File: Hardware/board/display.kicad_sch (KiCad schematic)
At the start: 1 part, among them U4 HS35B01A

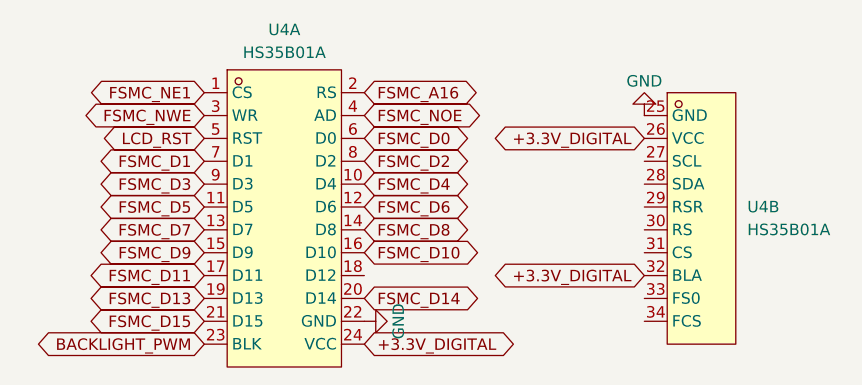
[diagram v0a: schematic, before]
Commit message: i am cooked
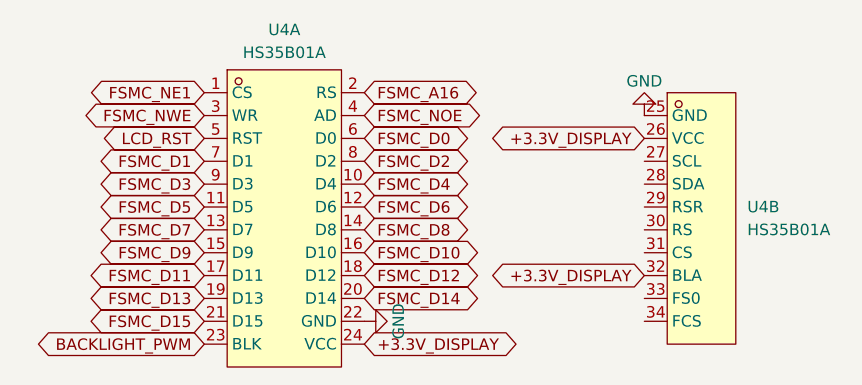
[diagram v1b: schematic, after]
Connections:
- net FSMC_D12: now reaches U4.18 (D12)
- net +3.3V_DIGITAL renamed +3.3V_DISPLAY
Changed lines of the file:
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@@
 	(generator_version "10.0")
 	(paper "A4")
+	(global_label "+3.3V_DISPLAY"
+		(shape bidirectional)
+		(at 146.05 51.435 180)
+		(effects
+			(font
+				(size 1.27 1.27)
+			)
+			(justify right)
+		)
+		(property "Intersheetrefs" "${INTERSHEET_REFS}"
+			(at 146.05 51.435 0)
+			(hide yes)
+			(show_name no)
+			(do_not_autoplace no)
+			(effects
+				(font
+					(size 1.27 1.27)
+				)
+			)
+		)
+	)
+	(global_label "+3.3V_DISPLAY"
+		(shape bidirectional)
+		(at 146.05 66.675 180)
+		(effects
+			(font
+				(size 1.27 1.27)
+			)
+			(justify right)
+		)
+		(property "Intersheetrefs" "${INTERSHEET_REFS}"
+			(at 146.05 66.675 0)
+			(hide yes)
+			(show_name no)
+			(do_not_autoplace no)
+			(effects
+				(font
+					(size 1.27 1.27)
+				)
+			)
+		)
+	)
 	(global_label "LCD_RST"
 		(shape bidirectional)
@@
 		)
 	)
-	(global_label "+3.3V_DIGITAL"
-		(shape bidirectional)
-		(at 146.05 51.435 180)
-		(effects
-			(font
-				(size 1.27 1.27)
-			)
-			(justify right)
-		)
-		(property "Intersheetrefs" "${INTERSHEET_REFS}"
-			(at 146.05 51.435 0)
-			(hide yes)
-			(show_name no)
-			(do_not_autoplace no)
-			(effects
-				(font
-					(size 1.27 1.27)
-				)
-			)
-		)
-	)
 	(global_label "FSMC_D14"
 		(shape bidirectional)
@@
 		)
 	)
+	(global_label "FSMC_D12"
+		(shape bidirectional)
+		(at 114.935 66.675 0)
+		(effects
+			(font
+				(size 1.27 1.27)
+			)
+			(justify left)
+		)
+		(property "Intersheetrefs" "${INTERSHEET_REFS}"
+			(at 114.935 66.675 0)
+			(hide yes)
+			(show_name no)
+			(do_not_autoplace no)
+			(effects
+				(font
+					(size 1.27 1.27)
+				)
+			)
+		)
+	)
 	(global_label "FSMC_NWE"
 		(shape bidirectional)
@@
 		)
 	)
-	(global_label "+3.3V_DIGITAL"
+	(global_label "FSMC_D4"
+		(shape bidirectional)
+		(at 114.935 56.515 0)
+		(effects
+			(font
+				(size 1.27 1.27)
+			)
+			(justify left)
+		)
+		(property "Intersheetrefs" "${INTERSHEET_REFS}"
+			(at 114.935 56.515 0)
+			(hide yes)
+			(show_name no)
+			(do_not_autoplace no)
+			(effects
+				(font
+					(size 1.27 1.27)
+				)
+			)
+		)
+	)
+	(global_label "+3.3V_DISPLAY"
 		(shape bidirectional)
 		(at 114.935 74.295 0)
@@
 		)
 	)
-	(global_label "FSMC_D4"
-		(shape bidirectional)
-		(at 114.935 56.515 0)
+	(global_label "FSMC_NE1"
+		(shape bidirectional)
+		(at 97.155 46.355 180)
+		(effects
+			(font
+				(size 1.27 1.27)
+			)
+			(justify right)
+		)
+		(property "Intersheetrefs" "${INTERSHEET_REFS}"
+			(at 97.155 46.355 0)
+			(hide yes)
+			(show_name no)
+			(do_not_autoplace no)
+			(effects
+				(font
+					(size 1.27 1.27)
+				)
+			)
+		)
+	)
+	(global_label "FSMC_D8"
+		(shape bidirectional)
+		(at 114.935 61.595 0)
 		(effects
 			(font
@@
 		)
 		(property "Intersheetrefs" "${INTERSHEET_REFS}"
-			(at 114.935 56.515 0)
-			(hide yes)
-			(show_name no)
-			(do_not_autoplace no)
-			(effects
-				(font
-					(size 1.27 1.27)
-				)
-			)
-		)
-	)
-	(global_label "FSMC_NE1"
-		(shape bidirectional)
-		(at 97.155 46.355 180)
-		(effects
-			(font
-				(size 1.27 1.27)
-			)
-			(justify right)
-		)
-		(property "Intersheetrefs" "${INTERSHEET_REFS}"
-			(at 97.155 46.355 0)
-			(hide yes)
-			(show_name no)
-			(do_not_autoplace no)
-			(effects
-				(font
-					(size 1.27 1.27)
-				)
-			)
-		)
-	)
-	(global_label "FSMC_D8"
-		(shape bidirectional)
-		(at 114.935 61.595 0)
+			(at 114.935 61.595 0)
+			(hide yes)
+			(show_name no)
+			(do_not_autoplace no)
+			(effects
+				(font
+					(size 1.27 1.27)
+				)
+			)
+		)
+	)
+	(global_label "BACKLIGHT_PWM"
+		(shape bidirectional)
+		(at 97.155 74.295 180)
+		(effects
+			(font
+				(size 1.27 1.27)
+			)
+			(justify right)
+		)
+		(property "Intersheetrefs" "${INTERSHEET_REFS}"
+			(at 97.155 74.295 0)
+			(hide yes)
+			(show_name no)
+			(do_not_autoplace no)
+			(effects
+				(font
+					(size 1.27 1.27)
+				)
+			)
+		)
+	)
+	(global_label "FSMC_A16"
+		(shape bidirectional)
+		(at 114.935 46.355 0)
 		(effects
 			(font
@@
 		)
 		(property "Intersheetrefs" "${INTERSHEET_REFS}"
-			(at 114.935 61.595 0)
-			(hide yes)
-			(show_name no)
-			(do_not_autoplace no)
-			(effects
-				(font
-					(size 1.27 1.27)
-				)
-			)
-		)
-	)
-	(global_label "BACKLIGHT_PWM"
-		(shape bidirectional)
-		(at 97.155 74.295 180)
-		(effects
-			(font
-				(size 1.27 1.27)
-			)
-			(justify right)
-		)
-		(property "Intersheetrefs" "${INTERSHEET_REFS}"
-			(at 97.155 74.295 0)
-			(hide yes)
-			(show_name no)
-			(do_not_autoplace no)
-			(effects
-				(font
-					(size 1.27 1.27)
-				)
-			)
-		)
-	)
-	(global_label "FSMC_A16"
-		(shape bidirectional)
-		(at 114.935 46.355 0)
-		(effects
-			(font
-				(size 1.27 1.27)
-			)
-			(justify left)
-		)
-		(property "Intersheetrefs" "${INTERSHEET_REFS}"
 			(at 114.935 46.355 0)
-			(hide yes)
-			(show_name no)
-			(do_not_autoplace no)
-			(effects
-				(font
-					(size 1.27 1.27)
-				)
-			)
-		)
-	)
-	(global_label "+3.3V_DIGITAL"
-		(shape bidirectional)
-		(at 146.05 66.675 180)
-		(effects
-			(font
-				(size 1.27 1.27)
-			)
-			(justify right)
-		)
-		(property "Intersheetrefs" "${INTERSHEET_REFS}"
-			(at 146.05 66.675 0)
 			(hide yes)
 			(show_name no)
@@
 		(dnp no)
 		(fields_autoplaced yes)
-		(property "Reference" "#PWR019"
+		(property "Reference" "#PWR022"
 			(at 121.285 71.755 0)
 			(hide yes)
@@
 			(project "board"
 				(path "/a701f4fd-d5c8-4ab0-b464-3edf07ec58ed/a518d5fa-3e63-4101-a721-9b8ba5303779"
-					(reference "#PWR019")
+					(reference "#PWR022")
 					(unit 1)
 				)
@@
 		(dnp no)
 		(fields_autoplaced yes)
-		(property "Reference" "#PWR018"
+		(property "Reference" "#PWR023"
 			(at 146.05 42.545 0)
 			(hide yes)
@@
 			(project "board"
 				(path "/a701f4fd-d5c8-4ab0-b464-3edf07ec58ed/a518d5fa-3e63-4101-a721-9b8ba5303779"
-					(reference "#PWR018")
+					(reference "#PWR023")
 					(unit 1)
 				)
